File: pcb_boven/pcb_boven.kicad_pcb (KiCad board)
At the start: 2 copper layers, 30 parts, among them U1 miniIMU-9_v6, U2 openMV_M7_R2

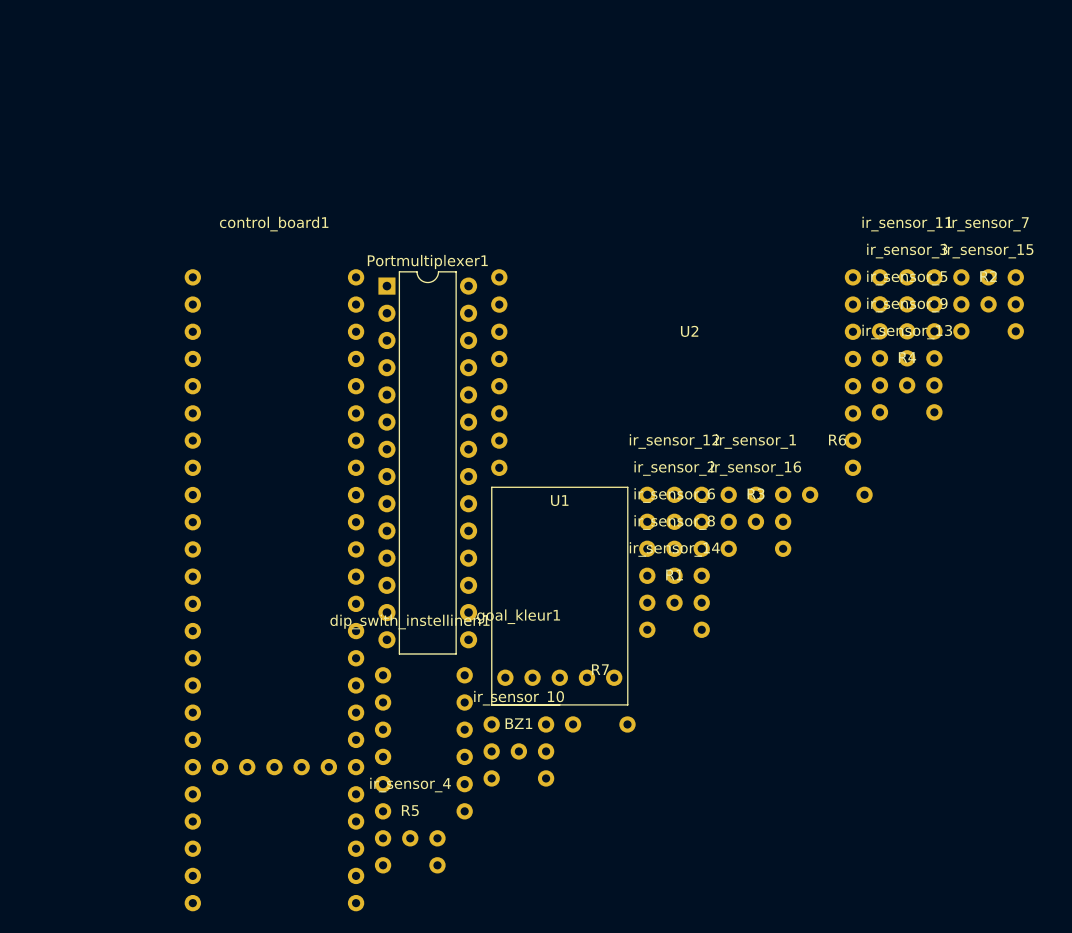
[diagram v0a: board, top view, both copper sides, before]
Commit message: pcb onder gemaakt
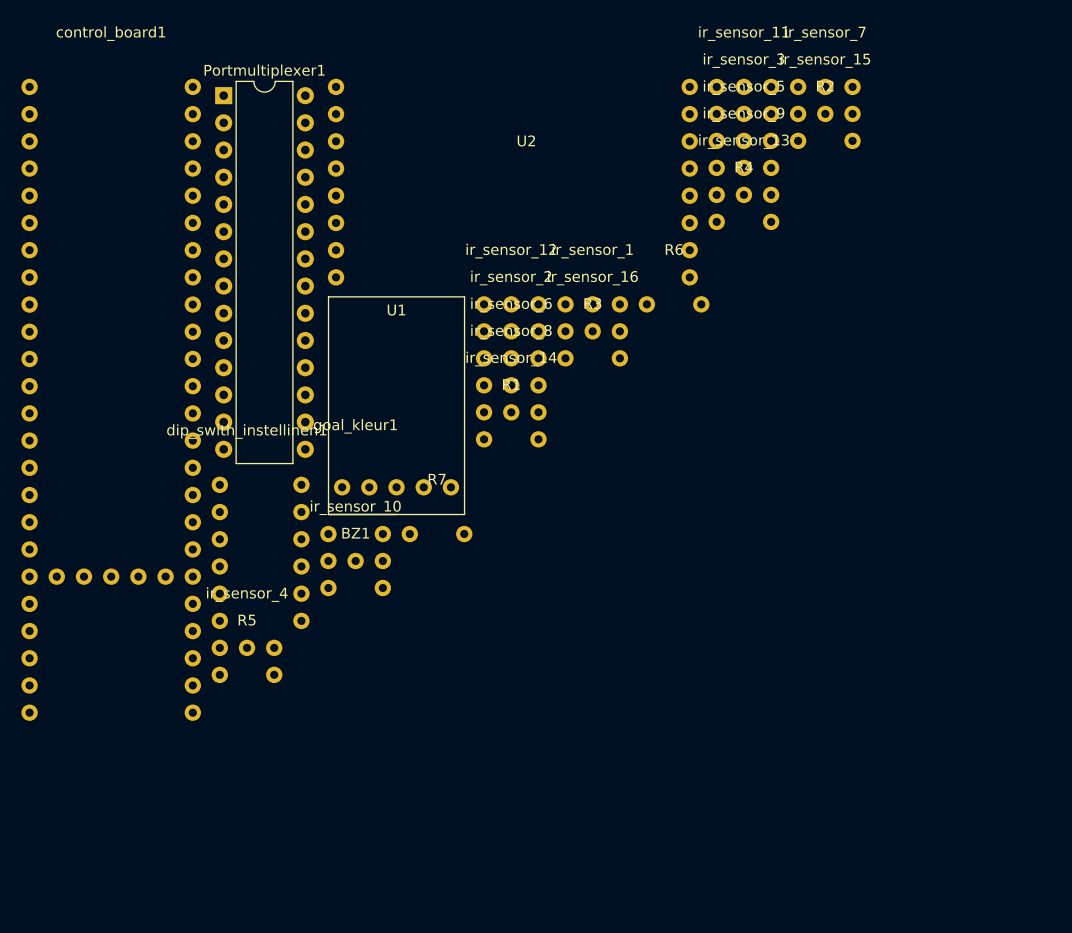
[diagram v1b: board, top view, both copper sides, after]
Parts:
- moved R1 23.4 mm to (145.3, 104.2)
- moved R2 23.4 mm to (174.7, 76.4)
- moved R3 23.4 mm to (152.9, 96.7)
- moved R6 23.4 mm to (160.5, 91.6)
- moved R7 23.4 mm to (138.4, 113.1)
- moved control_board1 23.4 mm to (108.0, 79.0)
- moved goal_kleur1 23.4 mm to (130.8, 113.1)
- moved ir_sensor_1 23.4 mm to (152.9, 91.6)
- moved ir_sensor_10 23.4 mm to (130.8, 115.6)
- moved ir_sensor_11 23.4 mm to (167.1, 71.3)
- moved ir_sensor_12 23.4 mm to (145.3, 91.6)
- moved ir_sensor_13 23.4 mm to (167.1, 81.4)
- moved ir_sensor_14 23.4 mm to (145.3, 101.7)
- moved ir_sensor_15 23.4 mm to (174.7, 73.8)
- moved ir_sensor_16 23.4 mm to (152.9, 94.2)
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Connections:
- ir_sensor_1 pad 1: Net-(ir_sensor_1-Pad1) -> 3.3v
- ir_sensor_1 pad 2: Net-(ir_sensor_1-Pad2) -> gnd
- ir_sensor_10 pad 1: Net-(ir_sensor_1-Pad1) -> 3.3v
- ir_sensor_10 pad 2: Net-(ir_sensor_1-Pad2) -> gnd
- ir_sensor_11 pad 1: Net-(ir_sensor_1-Pad1) -> 3.3v
- ir_sensor_11 pad 2: Net-(ir_sensor_1-Pad2) -> gnd
- ir_sensor_12 pad 1: Net-(ir_sensor_1-Pad1) -> 3.3v
- ir_sensor_12 pad 2: Net-(ir_sensor_1-Pad2) -> gnd
- ir_sensor_13 pad 1: Net-(ir_sensor_1-Pad1) -> 3.3v
- ir_sensor_13 pad 2: Net-(ir_sensor_1-Pad2) -> gnd
- ir_sensor_14 pad 1: Net-(ir_sensor_1-Pad1) -> 3.3v
- ir_sensor_14 pad 2: Net-(ir_sensor_1-Pad2) -> gnd
- ir_sensor_15 pad 1: Net-(ir_sensor_1-Pad1) -> 3.3v
- ir_sensor_15 pad 2: Net-(ir_sensor_1-Pad2) -> gnd
- ir_sensor_16 pad 1: Net-(ir_sensor_1-Pad1) -> 3.3v
- ir_sensor_16 pad 2: Net-(ir_sensor_1-Pad2) -> gnd
- ir_sensor_2 pad 1: Net-(ir_sensor_1-Pad1) -> 3.3v
- ir_sensor_2 pad 2: Net-(ir_sensor_1-Pad2) -> gnd
- ir_sensor_3 pad 1: Net-(ir_sensor_1-Pad1) -> 3.3v
- ir_sensor_3 pad 2: Net-(ir_sensor_1-Pad2) -> gnd
- ir_sensor_4 pad 1: Net-(ir_sensor_1-Pad1) -> 3.3v
- ir_sensor_4 pad 2: Net-(ir_sensor_1-Pad2) -> gnd
- ir_sensor_5 pad 1: Net-(ir_sensor_1-Pad1) -> 3.3v
- ir_sensor_5 pad 2: Net-(ir_sensor_1-Pad2) -> gnd
- ir_sensor_6 pad 1: Net-(ir_sensor_1-Pad1) -> 3.3v
- ir_sensor_6 pad 2: Net-(ir_sensor_1-Pad2) -> gnd
- ir_sensor_7 pad 1: Net-(ir_sensor_1-Pad1) -> 3.3v
- ir_sensor_7 pad 2: Net-(ir_sensor_1-Pad2) -> gnd
- ir_sensor_8 pad 1: Net-(ir_sensor_1-Pad1) -> 3.3v
- ir_sensor_8 pad 2: Net-(ir_sensor_1-Pad2) -> gnd
- ir_sensor_9 pad 1: Net-(ir_sensor_1-Pad1) -> 3.3v
- ir_sensor_9 pad 2: Net-(ir_sensor_1-Pad2) -> gnd

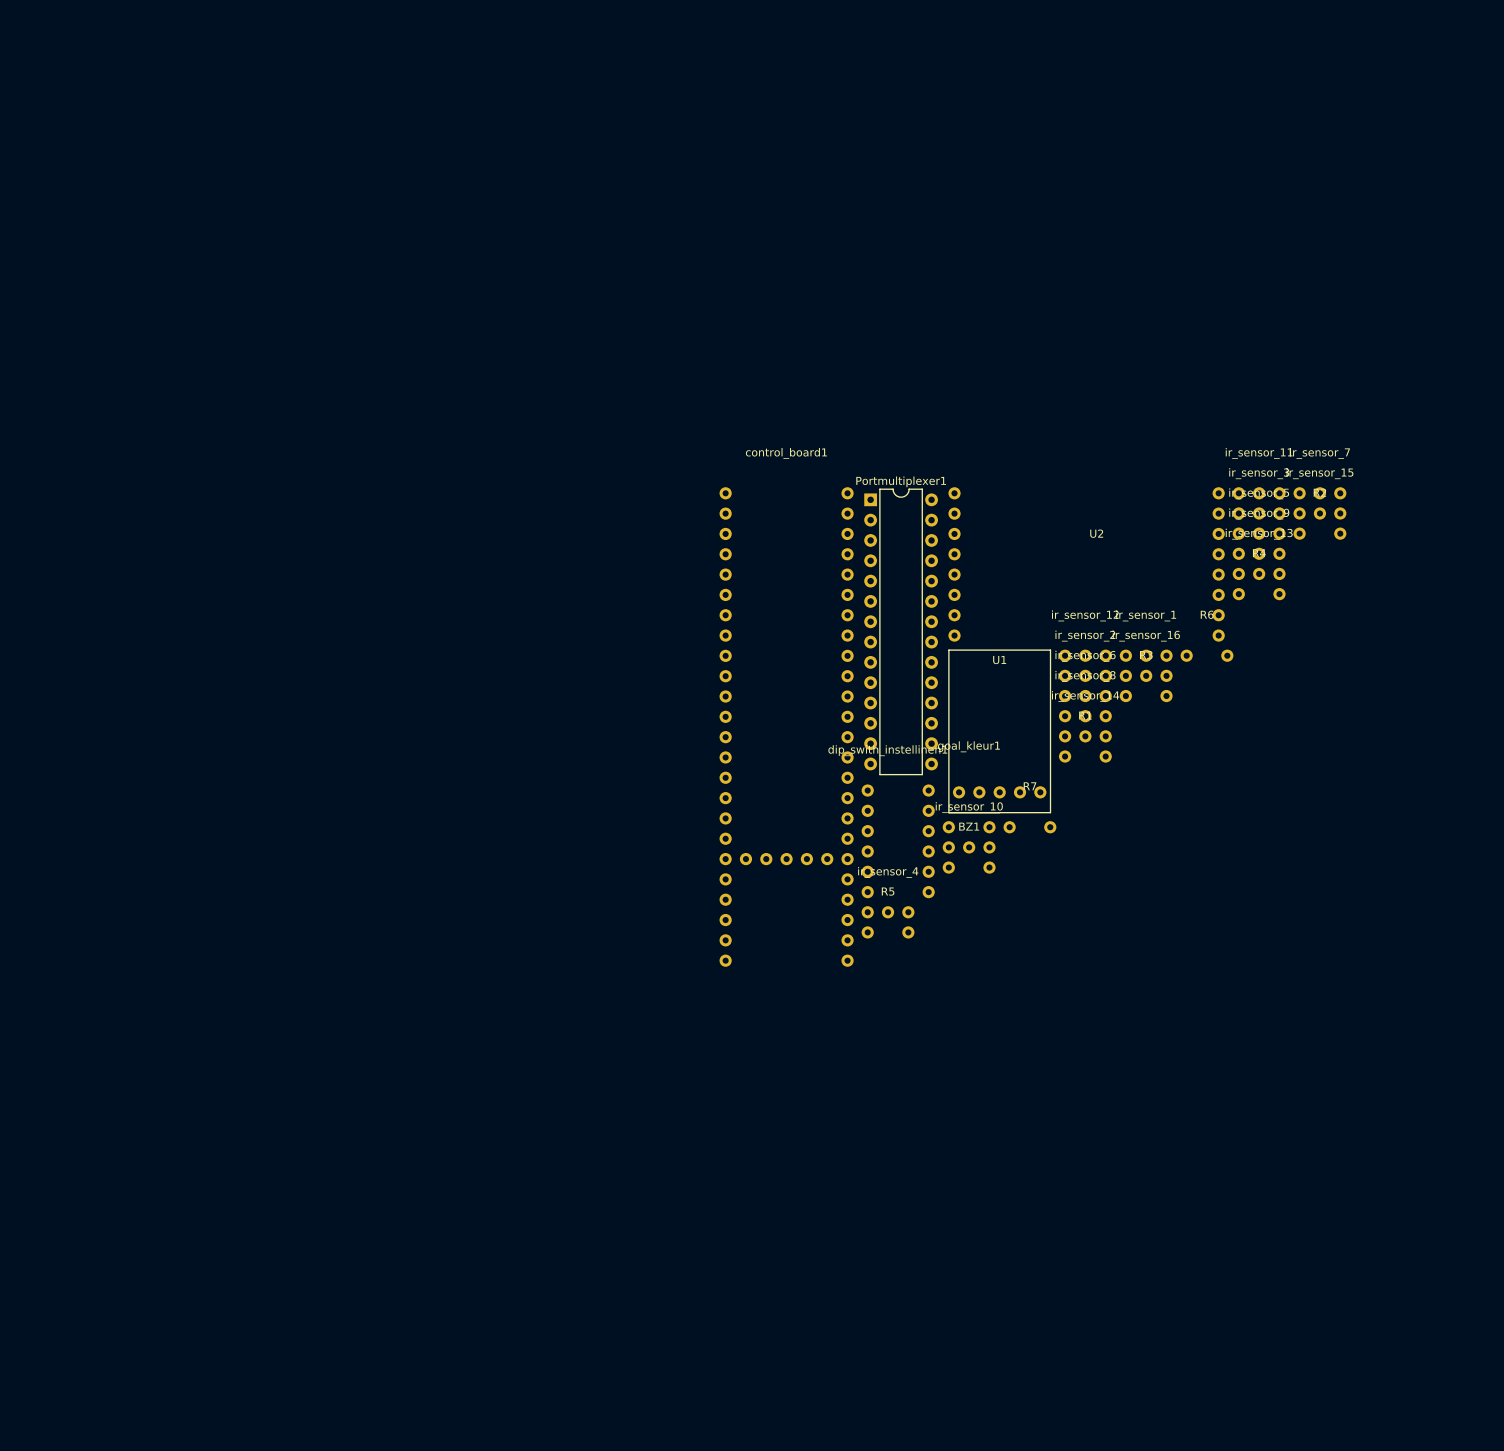
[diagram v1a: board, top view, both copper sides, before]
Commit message: pcb
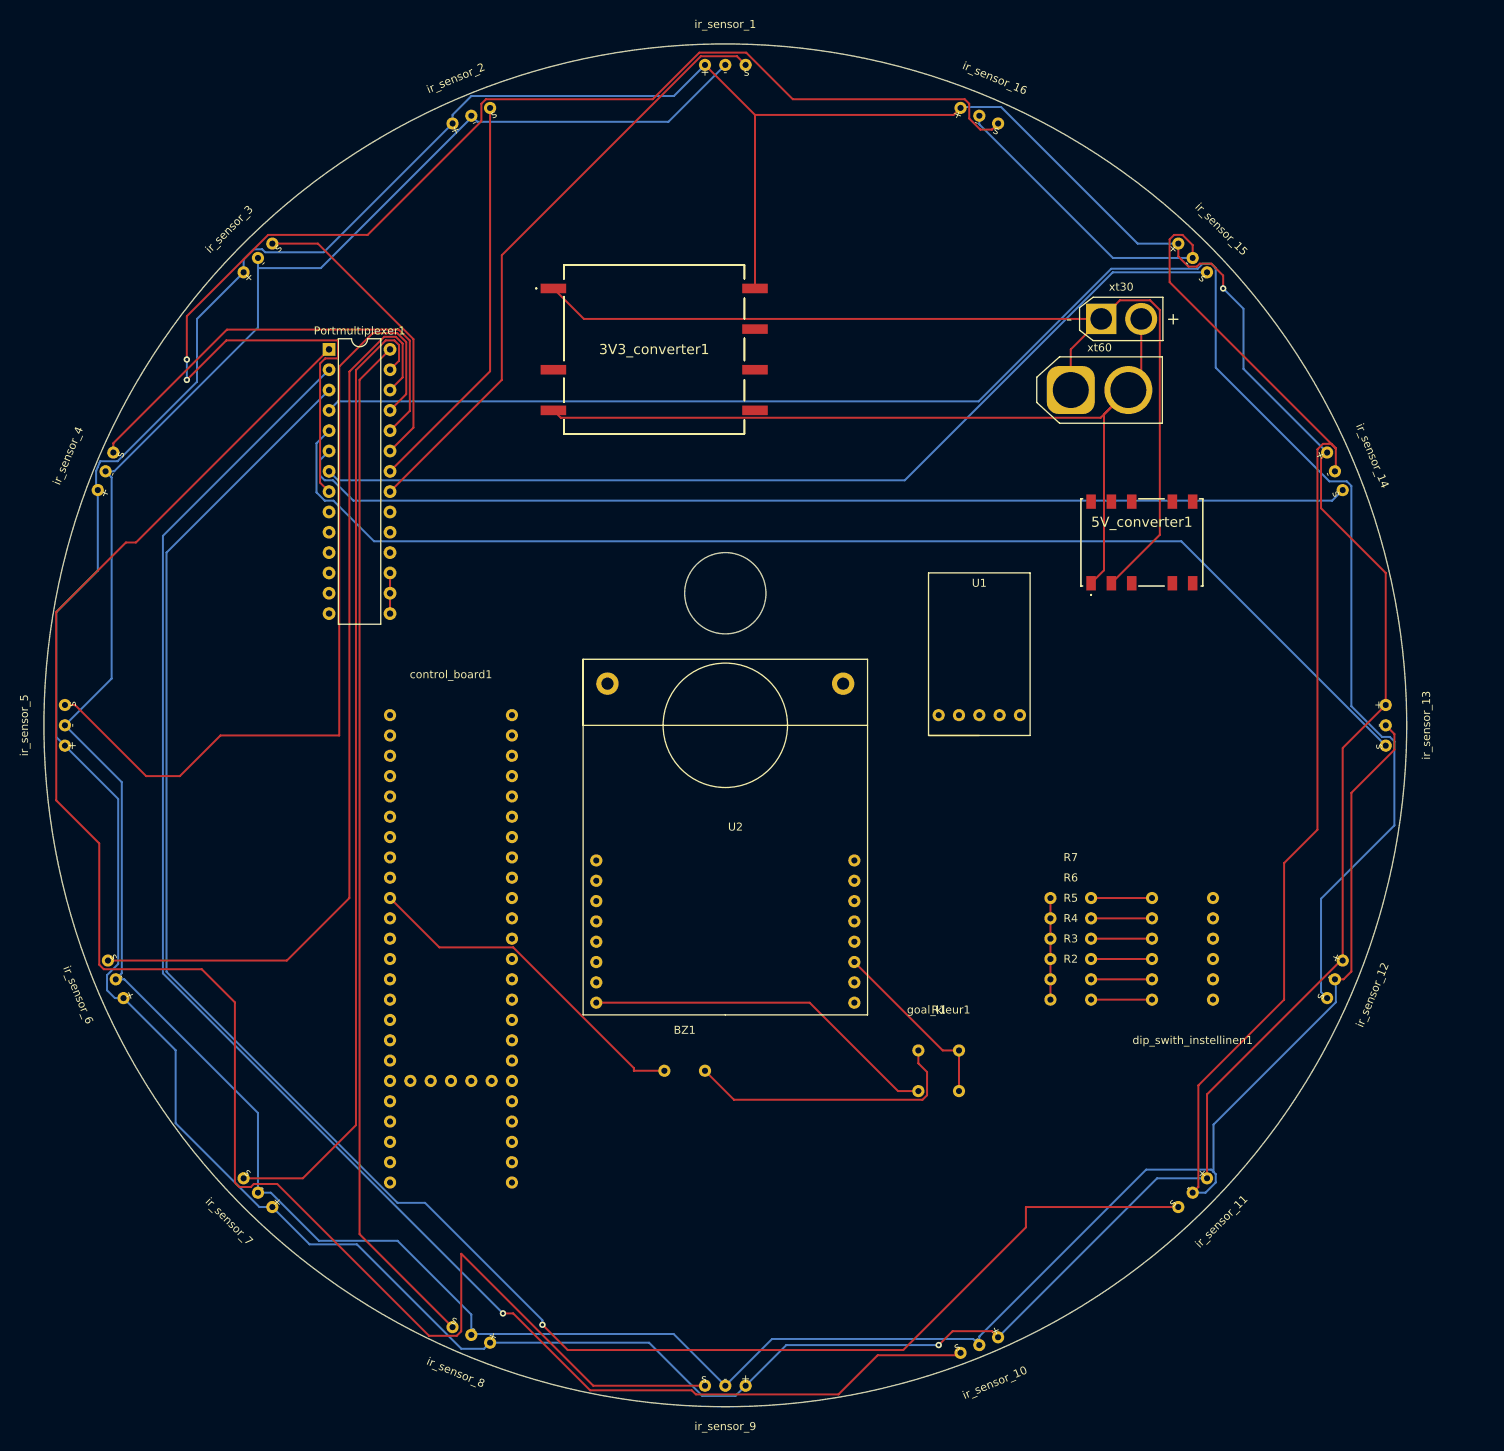
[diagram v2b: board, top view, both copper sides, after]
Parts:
- added 3V3_converter1: CC6-1203SR-E, custom:CC60512SRE, F.Cu at (91.4, 53.3)
- added 5V_converter1: SFTN01M-05N, custom:SFTN01M05N, F.Cu at (152.4, 77.5)
- added xt30: Battery, Connector_AMASS:AMASS_XT30U-F_1x02_P5.0mm_Vertical, F.Cu at (147.3, 49.5)
- added xt60: Battery, Connector_AMASS:AMASS_XT60-F_1x02_P7.20mm_Vertical, F.Cu at (143.5, 58.4)
- moved ir_sensor_7 158.9 mm to (41.9, 158.8), turned to 135 degrees
- moved ir_sensor_5 151.2 mm to (17.8, 100.3), turned to 90 degrees
- moved ir_sensor_3 129.2 mm to (41.9, 41.9), turned to 45 degrees
- moved ir_sensor_6 126.3 mm to (24.1, 132.1), turned to 112.5 degrees
- moved ir_sensor_9 123.6 mm to (100.3, 182.9), turned to 180 degrees
- moved ir_sensor_4 112.3 mm to (22.9, 68.6), turned to 67.5 degrees
- moved ir_sensor_8 109.0 mm to (68.6, 176.5), turned to 157.5 degrees
- moved ir_sensor_2 103.9 mm to (68.6, 24.1), turned to 22.5 degrees
- moved ir_sensor_1 90.7 mm to (100.3, 17.8)
- moved ir_sensor_11 87.8 mm to (158.8, 158.8), turned to 225 degrees
- moved ir_sensor_16 73.1 mm to (132.1, 24.1), turned to 337.5 degrees
- moved Portmultiplexer1 70.3 mm to (50.8, 53.3)
- moved R2 66.1 mm to (143.5, 134.6)
- moved ir_sensor_10 62.2 mm to (132.1, 177.8), turned to 202.5 degrees
- moved U2 58.1 mm to (100.3, 114.3)
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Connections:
- Portmultiplexer1 pad 15: Net-(Portmultiplexer1-Pad15) -> gnd
- Portmultiplexer1 pad 16: Net-(Portmultiplexer1-Pad16) -> gnd
- Portmultiplexer1 pad 17: Net-(Portmultiplexer1-Pad17) -> gnd
- control_board1 pad 12: A -> Net-(U2-Pad5)
- control_board1 pad 13: Net-(control_board1-Pad13) -> Net-(U2-Pad2)
- control_board1 pad 14: Net-(control_board1-Pad14) -> Net-(U2-Pad3)
- control_board1 pad 16: Net-(control_board1-Pad16) -> A
- control_board1 pad 2: Net-(control_board1-Pad2) -> scl
- control_board1 pad 28: Net-(control_board1-Pad28) -> Net-(U2-Pad4)
- control_board1 pad 3: Net-(control_board1-Pad3) -> sda
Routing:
- net gnd: track 0.00 -> 657.0 mm
- net 3.3v: track 0.00 -> 626.8 mm, vias 0 -> 2
- net Net-(Portmultiplexer1-Pad3): track 0.00 -> 236.4 mm, vias 0 -> 1
- net Net-(Portmultiplexer1-Pad4): track 0.00 -> 225.1 mm
- net Net-(Portmultiplexer1-Pad1): track 0.00 -> 219.2 mm
- net Net-(Portmultiplexer1-Pad2): track 0.00 -> 207.9 mm, vias 0 -> 1
- net Net-(Portmultiplexer1-Pad8): track 0.00 -> 171.8 mm, vias 0 -> 2
- net Net-(Portmultiplexer1-Pad5): track 0.00 -> 155.1 mm
- net Net-(Portmultiplexer1-Pad6): track 0.00 -> 133.2 mm
- net Net-(Portmultiplexer1-Pad28): track 0.00 -> 128.6 mm
- net Net-(3V3_converter1-Pad1): track 0.00 -> 126.0 mm
- net Net-(Portmultiplexer1-Pad27): track 0.00 -> 121.9 mm
- net Net-(Portmultiplexer1-Pad7): track 0.00 -> 121.0 mm
- net Net-(Portmultiplexer1-Pad26): track 0.00 -> 114.5 mm
- net Net-(3V3_converter1-Pad3): track 0.00 -> 109.3 mm
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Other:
- board outline added: 170.4 x 170.4 mm
